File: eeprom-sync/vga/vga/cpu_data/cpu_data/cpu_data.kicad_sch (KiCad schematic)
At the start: 32 parts, among them J1 Conn_02x06_Odd_Even, J10 Conn_01x03_Female, J11 Conn_01x02_Female, J12 Conn_02x05_Odd_Even, J2 Conn_01x02_Female, J3 Conn_01x04_Female, J4 Conn_01x15_Female, J5 Conn_01x15_Female, J6 Conn_02x08_Odd_Even, J7 Conn_01x02_Female, J8 Conn_01x02_Female, J9 Conn_01x08_Female, U1 GAL22V10, U2 74HC14, U3 74LS02, U4 IDT7205L12JG, U5 74LS573

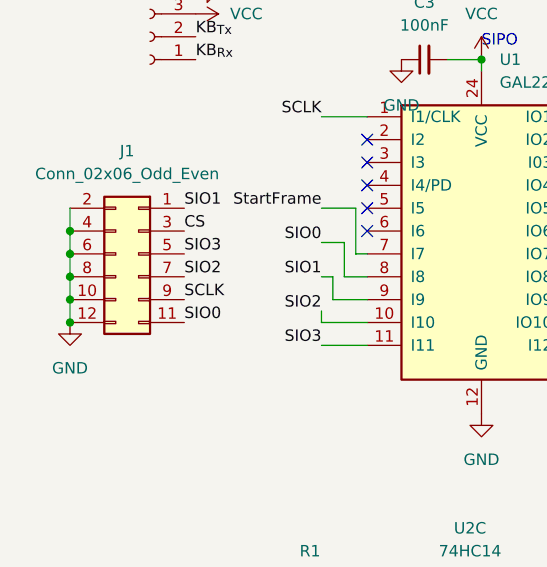
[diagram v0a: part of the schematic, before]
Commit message: routing completed
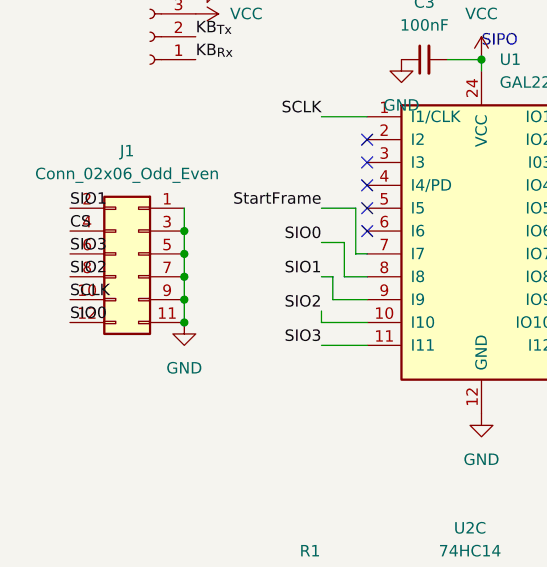
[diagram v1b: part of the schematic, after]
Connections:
- net CS: now also J1.4 (Pin_4); no longer J1.3 (Pin_3)
- net GND: now also J1.1 (Pin_1), J1.11 (Pin_11), J1.3 (Pin_3), J1.5 (Pin_5), J1.7 (Pin_7), J1.9 (Pin_9); no longer J1.10 (Pin_10), J1.12 (Pin_12), J1.2 (Pin_2), J1.4 (Pin_4), J1.6 (Pin_6), J1.8 (Pin_8)
- net SCLK: now also J1.10 (Pin_10); no longer J1.9 (Pin_9)
- net SIO0: now also J1.12 (Pin_12); no longer J1.11 (Pin_11)
- net SIO1: now also J1.2 (Pin_2); no longer J1.1 (Pin_1)
- net SIO2: now also J1.8 (Pin_8); no longer J1.7 (Pin_7)
- net SIO3: now also J1.6 (Pin_6); no longer J1.5 (Pin_5)
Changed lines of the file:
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@@
   (junction (at 116.84 109.22) (diameter 0) (color 0 0 0 0)
   )
-  (junction (at 13.97 107.95) (diameter 0) (color 0 0 0 0)
+  (junction (at 26.67 107.95) (diameter 0) (color 0 0 0 0)
   )
   (junction (at 167.64 148.59) (diameter 0) (color 0 0 0 0)
@@
   (junction (at 90.17 107.95) (diameter 0) (color 0 0 0 0)
   )
-  (junction (at 13.97 105.41) (diameter 0) (color 0 0 0 0)
-  )
-  (junction (at 13.97 110.49) (diameter 0) (color 0 0 0 0)
+  (junction (at 26.67 105.41) (diameter 0) (color 0 0 0 0)
+  )
+  (junction (at 26.67 110.49) (diameter 0) (color 0 0 0 0)
   )
   (junction (at 200.66 148.59) (diameter 0) (color 0 0 0 0)
   )
-  (junction (at 13.97 115.57) (diameter 0) (color 0 0 0 0)
-  )
-  (junction (at 13.97 113.03) (diameter 0) (color 0 0 0 0)
+  (junction (at 26.67 115.57) (diameter 0) (color 0 0 0 0)
+  )
+  (junction (at 26.67 113.03) (diameter 0) (color 0 0 0 0)
   )
   (junction (at 167.64 143.51) (diameter 0) (color 0 0 0 0)
@@
     (stroke (width 0) (type default) (color 0 0 0 0))
   )
-  (wire (pts (xy 13.97 105.41) (xy 13.97 107.95))
+  (wire (pts (xy 26.67 105.41) (xy 26.67 107.95))
     (stroke (width 0) (type default) (color 0 0 0 0))
   )
@@
     (stroke (width 0) (type default) (color 0 0 0 0))
   )
-  (wire (pts (xy 13.97 110.49) (xy 13.97 113.03))
+  (wire (pts (xy 26.67 110.49) (xy 26.67 113.03))
     (stroke (width 0) (type default) (color 0 0 0 0))
   )
@@
     (stroke (width 0) (type default) (color 0 0 0 0))
   )
-  (wire (pts (xy 13.97 107.95) (xy 13.97 110.49))
+  (wire (pts (xy 26.67 107.95) (xy 26.67 110.49))
     (stroke (width 0) (type default) (color 0 0 0 0))
   )
@@
     (stroke (width 0) (type default) (color 0 0 0 0))
   )
-  (wire (pts (xy 13.97 113.03) (xy 13.97 115.57))
+  (wire (pts (xy 26.67 113.03) (xy 26.67 115.57))
     (stroke (width 0) (type default) (color 0 0 0 0))
   )
@@
     (stroke (width 0) (type default) (color 0 0 0 0))
   )
-  (wire (pts (xy 13.97 102.87) (xy 13.97 105.41))
+  (wire (pts (xy 26.67 102.87) (xy 26.67 105.41))
     (stroke (width 0) (type default) (color 0 0 0 0))
   )
@@
     (effects (font (size 1.27 1.27)) (justify left bottom))
   )
-  (label "SIO0" (at 26.67 115.57 0)
+  (label "SIO0" (at 13.97 115.57 0)
     (effects (font (size 1.27 1.27)) (justify left bottom))
   )
@@
     (effects (font (size 1.27 1.27)) (justify right bottom))
   )
-  (label "SIO2" (at 26.67 110.49 0)
+  (label "SIO2" (at 13.97 110.49 0)
     (effects (font (size 1.27 1.27)) (justify left bottom))
   )
@@
     (effects (font (size 1.27 1.27)) (justify right bottom))
   )
-  (label "SIO1" (at 26.67 102.87 0)
-    (effects (font (size 1.27 1.27)) (justify left bottom))
-  )
-  (label "SCLK" (at 26.67 113.03 0)
+  (label "SIO1" (at 13.97 102.87 0)
+    (effects (font (size 1.27 1.27)) (justify left bottom))
+  )
+  (label "SCLK" (at 13.97 113.03 0)
     (effects (font (size 1.27 1.27)) (justify left bottom))
   )
@@
     (effects (font (size 1.27 1.27)) (justify left bottom))
   )
-  (label "SIO3" (at 26.67 107.95 0)
+  (label "SIO3" (at 13.97 107.95 0)
     (effects (font (size 1.27 1.27)) (justify left bottom))
   )
@@
     (effects (font (size 1.27 1.27)) (justify left bottom))
   )
-  (label "CS" (at 26.67 105.41 0)
+  (label "CS" (at 13.97 105.41 0)
     (effects (font (size 1.27 1.27)) (justify left bottom))
   )
@@
     (pin "2")
   )
-  (symbol (lib_id "power:GND") (at 13.97 115.57 0) (unit 1)
-    (in_bom yes) (on_board yes) (fields_autoplaced)
-    (property "Reference" "#PWR0104" (id 0) (at 13.97 121.92 0)
-      (effects (font (size 1.27 1.27)) hide)
-    )
-    (property "Value" "GND" (id 1) (at 13.97 120.65 0))
-    (property "Footprint" "" (id 2) (at 13.97 115.57 0)
-      (effects (font (size 1.27 1.27)) hide)
-    )
-    (property "Datasheet" "" (id 3) (at 13.97 115.57 0)
-      (effects (font (size 1.27 1.27)) hide)
-    )
+  (symbol (lib_id "power:GND") (at 26.67 115.57 0) (unit 1)
+    (in_bom yes) (on_board yes) (fields_autoplaced)
+    (property "Reference" "#PWR0104" (id 0) (at 26.67 121.92 0)
+      (effects (font (size 1.27 1.27)) hide)
+    )
+    (property "Value" "GND" (id 1) (at 26.67 120.65 0))
+    (property "Footprint" "" (id 2) (at 26.67 115.57 0)
+      (effects (font (size 1.27 1.27)) hide)
+    )
+    (property "Datasheet" "" (id 3) (at 26.67 115.57 0)
+      (effects (font (size 1.27 1.27)) hide)
+    )
